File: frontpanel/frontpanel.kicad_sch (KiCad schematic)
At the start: 1 part

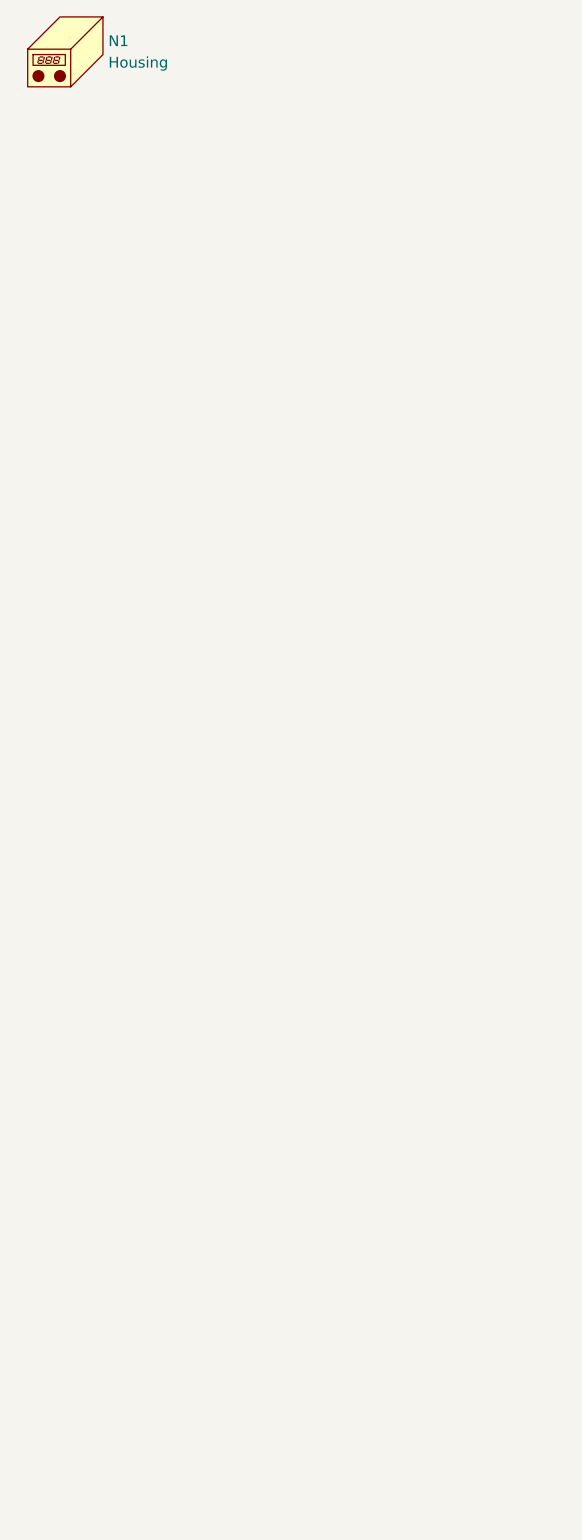
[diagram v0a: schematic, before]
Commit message: Work in progress
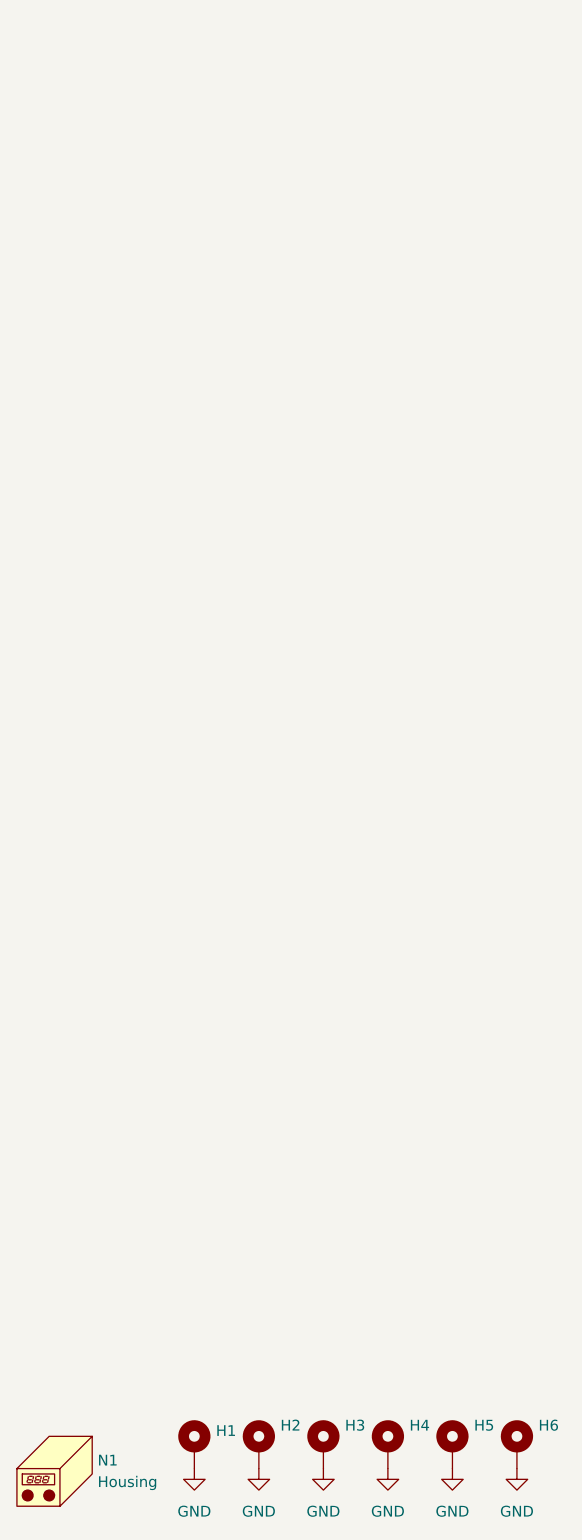
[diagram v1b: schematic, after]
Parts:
- added H1, H2, H3, H4, H5, H6: ~, MountingHole:MountingHole_2.2mm_M2_Pad_Via, symbol Mechanical:MountingHole_Pad
- N1: footprint proto1_kicad_art:proto1_kicad_art -> design:proto1_kicad_art2
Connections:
- new net GND: H1.1, H2.1, H3.1, H4.1, H5.1, H6.1
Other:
- company: (none) -> Badge.Team
- title: (none) -> WHY2025 badge
